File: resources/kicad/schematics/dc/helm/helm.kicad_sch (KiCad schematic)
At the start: 210 parts, among them J1 20, J146 02, J147 05, J148 03, J149 01, J150 02, J151 05, J152 06, J153 09, J155 10, J156 15, J157 14, J158 16, J159 20, J160 21, J161 08, J162 25, J163 38, J164 39, J165 13, J166 32, J167 11, J168 40, J169 09, J170 41, J171 43, J172 44, J173 49, J174 51, J175 18, J176 19, J177 04, J178 53, J179 10, J180 20, J181 55, J182 56, J183 46, J184 47, J185 45, J187 01, J188 12, J189 36, J190 37, J191 62, J192 13, J193 48, J194 07, J195 14, J196 42, J197 31, J198 33, J2 42, J200 02, J201 03, J202 04, J203 05, J204 34, J205 06, J206 35, J207 07, J208 24, J209 52, J210 28, J211 11, J212 23, J213 10, J214 29, J215 30, J216 26, J217 27, J218 17, J219 22, J220 14, J221 21, J222 50, J223 15, J224 16, J225 15, J226 23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

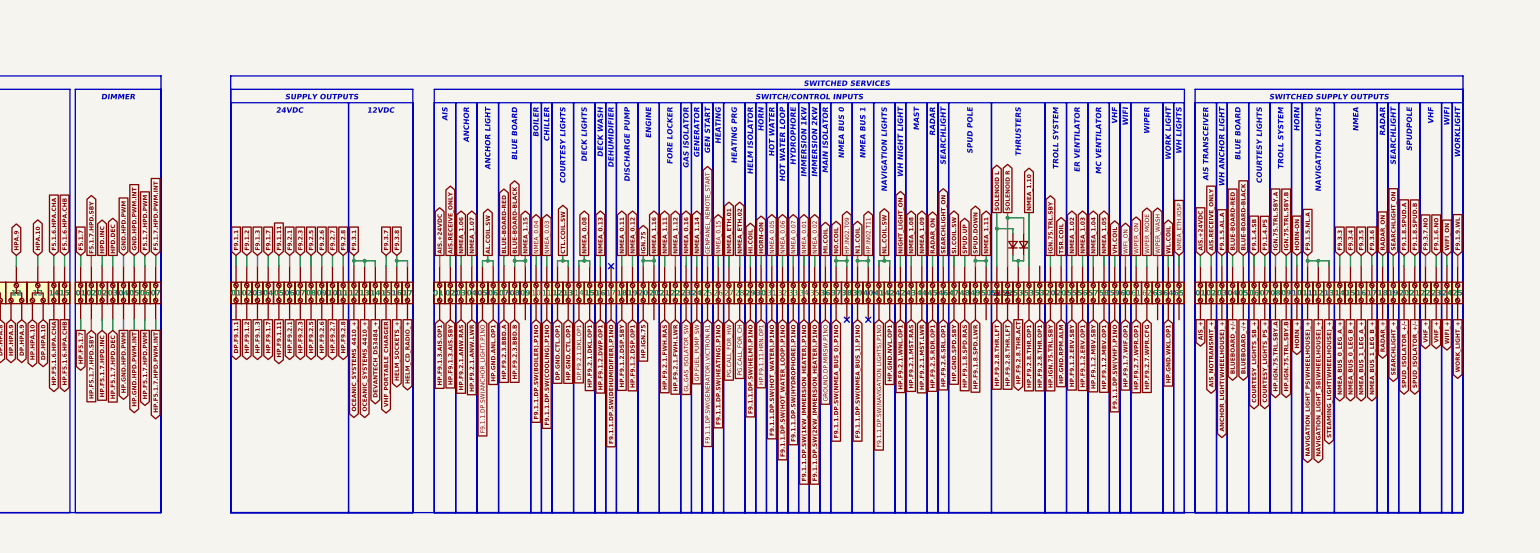
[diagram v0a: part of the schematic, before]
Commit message: Tidy up
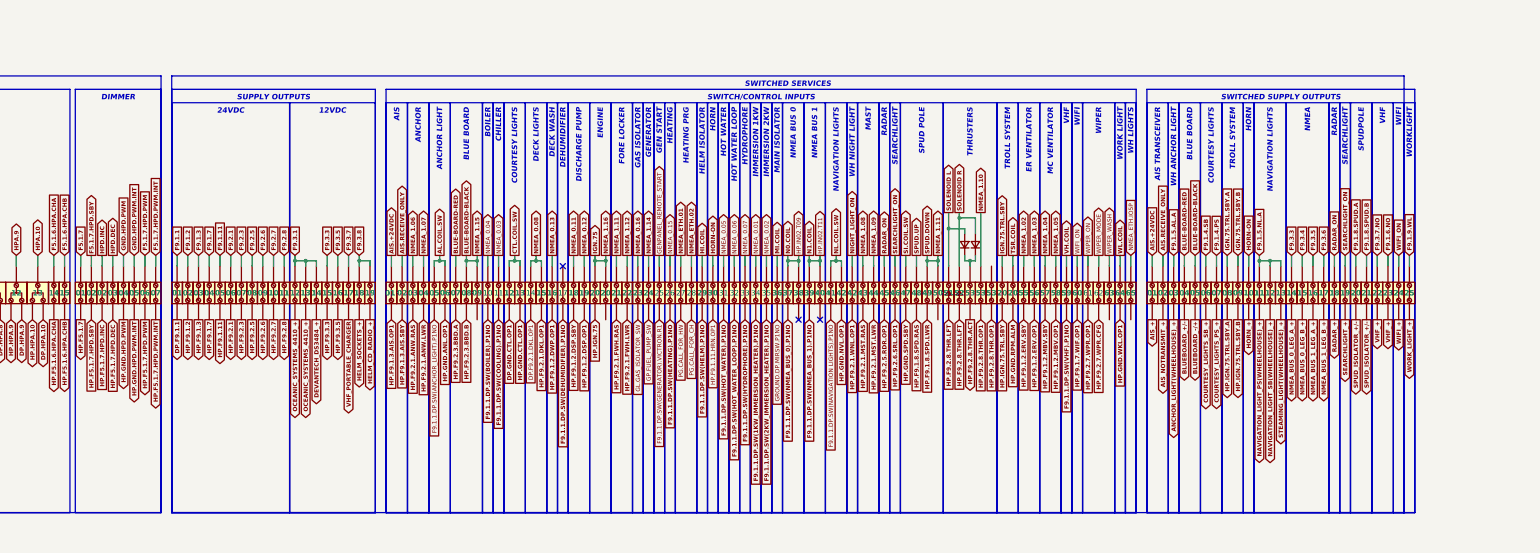
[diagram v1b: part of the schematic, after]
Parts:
- added J6: 15, symbol Beatrice:Conn_02x01_4MM2_BLUE
- added J7: 16, symbol Beatrice:Conn_02x01_4MM2_BLUE
- J225: value 15 -> 17
- J248: value 16 -> 18
- J249: value 17 -> 19
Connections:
- net F9.3.3: now also J6. (Pin_2)
- net F9.3.5: now also J7. (Pin_2)
- new net: J261. (Pin_2), J262. (Pin_2)
- new net: J266. (Pin_2), J269. (Pin_2)
- new net HP.F9.3.3: J6. (Pin_2)
- new net HP.F9.3.5: J7. (Pin_2)

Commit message: Reformat switch diagram
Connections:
- new net: J261. (Pin_2), J262. (Pin_2)
- new net: J266. (Pin_2), J269. (Pin_2)
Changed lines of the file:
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@@
 	)
 	(symbol
-		(lib_name "Beatrice:Conn_02x01_24VDC")
 		(lib_id "Beatrice:Conn_02x01_24VDC")
 		(at 236.22 350.52 90)
@@
 	)
 	(symbol
-		(lib_name "Beatrice:Conn_02x01_4MM2_GREY")
 		(lib_id "Beatrice:Conn_02x01_4MM2_GREY")
 		(at 373.38 350.52 90)
@@
 	)
 	(symbol
-		(lib_name "Beatrice:Conn_02x01_4MM2_GREY")
 		(lib_id "Beatrice:Conn_02x01_4MM2_GREY")
 		(at 365.76 350.52 90)
@@
 	)
 	(symbol
-		(lib_name "Beatrice:Conn_02x01_24VDC")
 		(lib_id "Beatrice:Conn_02x01_24VDC")
 		(at 292.1 350.52 90)
@@
 	)
 	(symbol
-		(lib_name "Beatrice:Conn_02x01_24VDC")
 		(lib_id "Beatrice:Conn_02x01_24VDC")
 		(at 269.24 350.52 90)
@@
 	)
 	(symbol
-		(lib_name "Beatrice:Conn_02x01_24VDC")
 		(lib_id "Beatrice:Conn_02x01_24VDC")
 		(at 226.06 350.52 90)
@@
 	)
 	(symbol
-		(lib_name "Beatrice:Conn_02x01_24VDC")
 		(lib_id "Beatrice:Conn_02x01_24VDC")
 		(at 287.02 350.52 90)
@@
 	)
 	(symbol
-		(lib_name "Beatrice:Conn_02x01_24VDC")
 		(lib_id "Beatrice:Conn_02x01_24VDC")
 		(at 243.84 350.52 90)
@@
 	)
 	(symbol
-		(lib_name "Beatrice:Conn_02x01_24VDC")
 		(lib_id "Beatrice:Conn_02x01_24VDC")
 		(at 271.78 350.52 90)
@@
 	)
 	(symbol
-		(lib_name "Beatrice:Conn_02x01_24VDC")
 		(lib_id "Beatrice:Conn_02x01_24VDC")
 		(at 284.48 350.52 90)
@@
 	)
 	(symbol
-		(lib_name "Beatrice:Conn_02x01_24VDC")
 		(lib_id "Beatrice:Conn_02x01_24VDC")
 		(at 289.56 350.52 90)
@@
 	)
 	(symbol
-		(lib_name "Beatrice:Conn_02x01_24VDC")
 		(lib_id "Beatrice:Conn_02x01_24VDC")
 		(at 228.6 350.52 90)
@@
 	)
 	(symbol
-		(lib_name "Beatrice:Conn_02x01_24VDC")
 		(lib_id "Beatrice:Conn_02x01_24VDC")
 		(at 266.7 350.52 90)
@@
 	)
 	(symbol
-		(lib_name "Beatrice:Conn_02x01_24VDC")
 		(lib_id "Beatrice:Conn_02x01_24VDC")
 		(at 368.3 350.52 90)
@@
 	)
 	(symbol
-		(lib_name "Beatrice:Conn_02x01_24VDC")
 		(lib_id "Beatrice:Conn_02x01_24VDC")
 		(at 274.32 350.52 90)
@@
 	)
 	(symbol
-		(lib_name "Beatrice:Conn_02x01_24VDC")
 		(lib_id "Beatrice:Conn_02x01_24VDC")
 		(at 281.94 350.52 90)
@@
 	)
 	(symbol
-		(lib_name "Beatrice:Conn_02x01_24VDC")
 		(lib_id "Beatrice:Conn_02x01_24VDC")
 		(at 370.84 350.52 90)
@@
 	)
 	(symbol
-		(lib_name "Beatrice:Conn_02x01_24VDC")
 		(lib_id "Beatrice:Conn_02x01_24VDC")
 		(at 213.36 350.52 90)
@@
 	)
 	(symbol
-		(lib_name "Beatrice:Conn_02x01_4MM2_GREY")
 		(lib_id "Beatrice:Conn_02x01_4MM2_GREY")
 		(at 378.46 350.52 90)

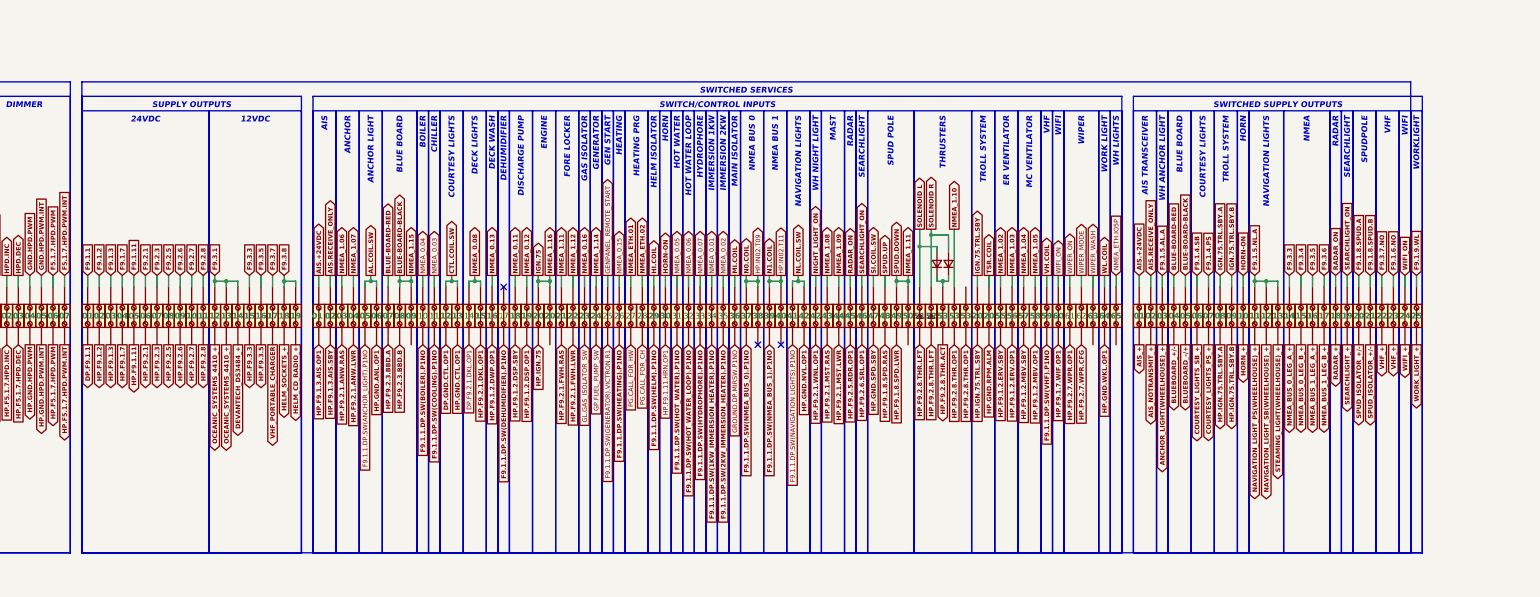
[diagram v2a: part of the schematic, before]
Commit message: Update helm.kicad_sch
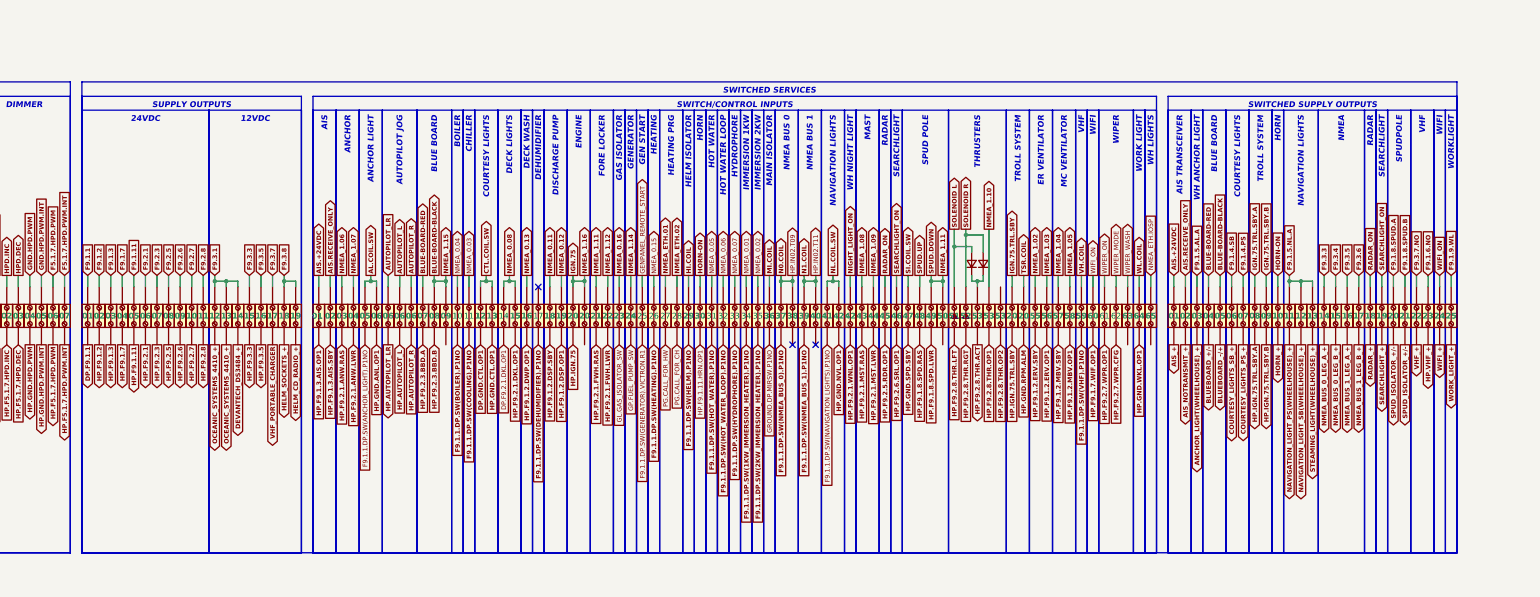
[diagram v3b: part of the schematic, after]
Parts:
- added J10, J8, J9: 06, symbol Beatrice:Conn_02x01_24VDC
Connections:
- net HP.F9.2.8.THR.LFT: no longer J209. (Pin_2)
- net HP.F9.2.8.THR.OP1: no longer J4. (Pin_2)
- net VHF_+: no longer J226. (Pin_2)
- net HP.F9.2.8.THR.OP2: now reaches J4. (Pin_2)
- new net: J261. (Pin_2), J262. (Pin_2)
- new net: J266. (Pin_2), J269. (Pin_2)
- new net AUTOPILOT_L: J9. (Pin_2)
- new net AUTOPILOT_LR: J8. (Pin_2)
- new net AUTOPILOT_R: J10. (Pin_2)
- new net HP.AUTOPILOT_L: J9. (Pin_2)
- new net HP.AUTOPILOT_LR: J8. (Pin_2)
- new net HP.AUTOPILOT_R: J10. (Pin_2)
- new net HP.F9.2.8.THR.RGT: J209. (Pin_2)
- new net HP.VHF_+: J226. (Pin_2)

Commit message: Add wire colors / sizes
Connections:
- new net: J261. (Pin_2), J262. (Pin_2)
- new net: J266. (Pin_2), J269. (Pin_2)
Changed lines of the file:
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@@
 	)
 	(symbol
-		(lib_name "Beatrice:Conn_02x01_24VDC")
 		(lib_id "Beatrice:Conn_02x01_24VDC")
 		(at 243.84 350.52 90)
@@
 	)
 	(symbol
-		(lib_name "Beatrice:Conn_02x01_4MM2_GREY")
 		(lib_id "Beatrice:Conn_02x01_4MM2_GREY")
 		(at 381 350.52 90)
@@
 	)
 	(symbol
-		(lib_name "Beatrice:Conn_02x01_4MM2_GREY")
 		(lib_id "Beatrice:Conn_02x01_4MM2_GREY")
 		(at 373.38 350.52 90)
@@
 	)
 	(symbol
-		(lib_name "Beatrice:Conn_02x01_24VDC")
 		(lib_id "Beatrice:Conn_02x01_24VDC")
 		(at 299.72 350.52 90)
@@
 	)
 	(symbol
-		(lib_name "Beatrice:Conn_02x01_24VDC")
 		(lib_id "Beatrice:Conn_02x01_24VDC")
 		(at 276.86 350.52 90)
@@
 	)
 	(symbol
-		(lib_name "Beatrice:Conn_02x01_24VDC")
 		(lib_id "Beatrice:Conn_02x01_24VDC")
 		(at 233.68 350.52 90)
@@
 	)
 	(symbol
-		(lib_name "Beatrice:Conn_02x01_24VDC")
 		(lib_id "Beatrice:Conn_02x01_24VDC")
 		(at 294.64 350.52 90)
@@
 	)
 	(symbol
-		(lib_name "Beatrice:Conn_02x01_24VDC")
 		(lib_id "Beatrice:Conn_02x01_24VDC")
 		(at 251.46 350.52 90)
@@
 	)
 	(symbol
-		(lib_name "Beatrice:Conn_02x01_24VDC")
 		(lib_id "Beatrice:Conn_02x01_24VDC")
 		(at 279.4 350.52 90)
@@
 	)
 	(symbol
-		(lib_name "Beatrice:Conn_02x01_24VDC")
 		(lib_id "Beatrice:Conn_02x01_24VDC")
 		(at 292.1 350.52 90)
@@
 	)
 	(symbol
-		(lib_name "Beatrice:Conn_02x01_24VDC")
 		(lib_id "Beatrice:Conn_02x01_24VDC")
 		(at 297.18 350.52 90)
@@
 	)
 	(symbol
-		(lib_name "Beatrice:Conn_02x01_24VDC")
 		(lib_id "Beatrice:Conn_02x01_24VDC")
 		(at 236.22 350.52 90)
@@
 	)
 	(symbol
-		(lib_name "Beatrice:Conn_02x01_24VDC")
 		(lib_id "Beatrice:Conn_02x01_24VDC")
 		(at 274.32 350.52 90)
@@
 	)
 	(symbol
-		(lib_name "Beatrice:Conn_02x01_24VDC")
 		(lib_id "Beatrice:Conn_02x01_24VDC")
 		(at 375.92 350.52 90)
@@
 	)
 	(symbol
-		(lib_name "Beatrice:Conn_02x01_24VDC")
 		(lib_id "Beatrice:Conn_02x01_24VDC")
 		(at 281.94 350.52 90)
@@
 	)
 	(symbol
-		(lib_name "Beatrice:Conn_02x01_24VDC")
 		(lib_id "Beatrice:Conn_02x01_24VDC")
 		(at 289.56 350.52 90)
@@
 	)
 	(symbol
-		(lib_name "Beatrice:Conn_02x01_24VDC")
 		(lib_id "Beatrice:Conn_02x01_24VDC")
 		(at 378.46 350.52 90)
@@
 	)
 	(symbol
-		(lib_name "Beatrice:Conn_02x01_24VDC")
 		(lib_id "Beatrice:Conn_02x01_24VDC")
 		(at 213.36 350.52 90)
@@
 	)
 	(symbol
-		(lib_name "Beatrice:Conn_02x01_4MM2_GREY")
 		(lib_id "Beatrice:Conn_02x01_4MM2_GREY")
 		(at 386.08 350.52 90)
